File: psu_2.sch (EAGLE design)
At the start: 32 parts, among them IC1 7812TV

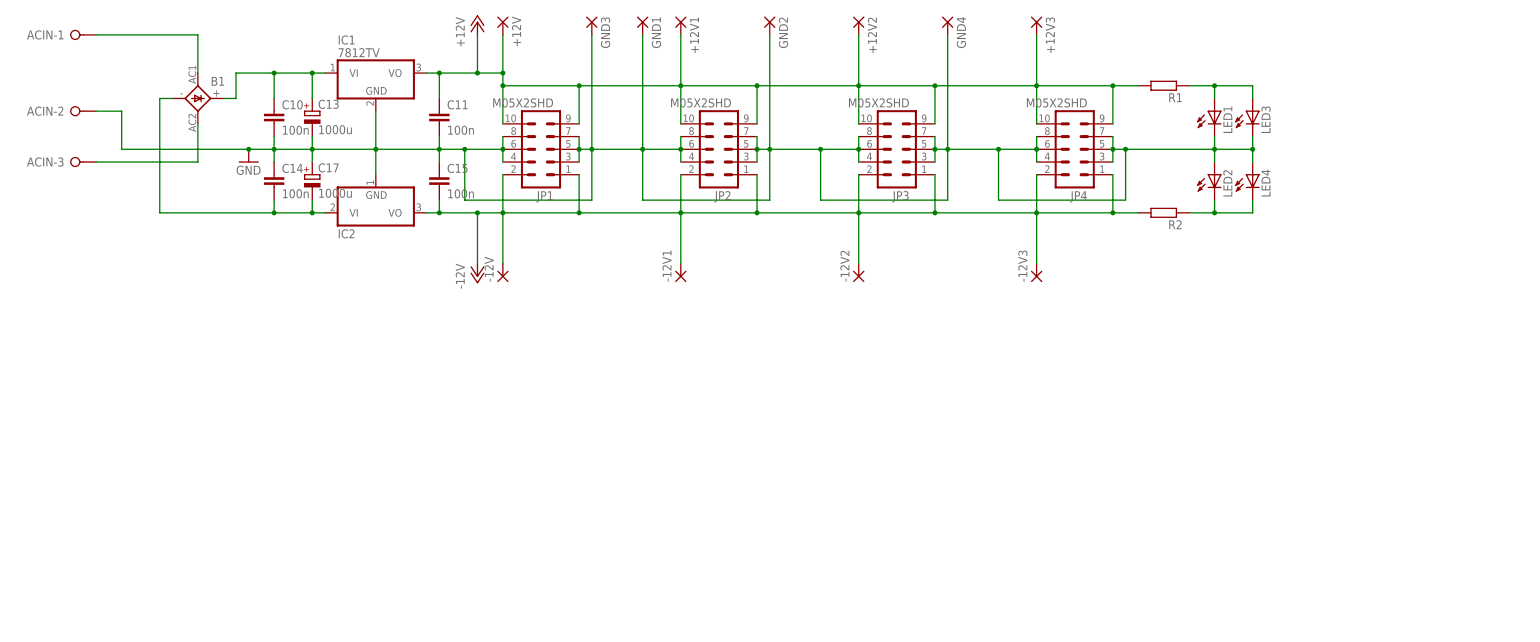
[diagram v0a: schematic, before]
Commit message: Add files via upload
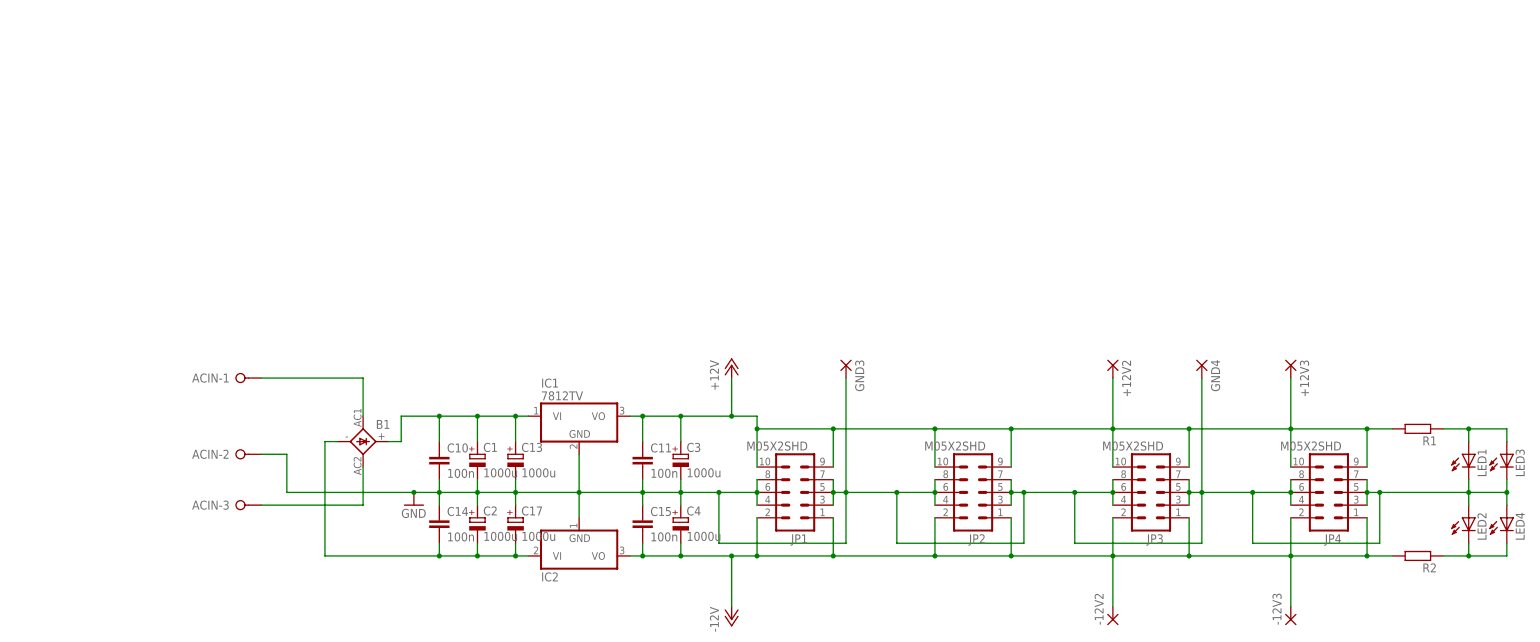
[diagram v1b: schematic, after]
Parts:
- removed +12V, +12V1, -12V, -12V1, GND1, GND2: (no value), wirepad:2,54/1,0
- added C1, C2, C3, C4: 1000u, rcl:CPOL-EUE3.5-10
- C13, C17: device rcl:CPOL-EUE3.5-8 -> rcl:CPOL-EUE3.5-10
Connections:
- net +12V: now also C3.+; no longer +12V.P, +12V1.P
- net -12V: now also C4.-; no longer -12V.P, -12V1.P
- net GND: now also C1.-, C2.+, C3.-, C4.+; no longer GND1.P, GND2.P
- net N$3: now also C2.-
- net N$4: now also C1.+
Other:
- moved on the sheet: +12V2, +12V3, -12V2, -12V3, ACIN-1, ACIN-2, ACIN-3, B1, C10, C11, C13, C14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
